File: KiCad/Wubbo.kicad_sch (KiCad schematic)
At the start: 43 parts, among them J1 USB_C_Receptacle, J2 SWD, J3 USB, J4 JST-BATT, Q1 AO3407, Q2 AO3407, SW1 Choc, SW10 Choc, SW11 Choc, SW12 Choc, SW13 Choc, SW14 Choc, SW15 Choc, SW16 Choc, SW17 Choc, SW2 Choc, SW3 Choc, SW4 Choc, SW5 Choc, SW6 Choc, SW7 Choc, SW8 Choc, SW9 Choc, U1 nRF52840_holyiot_18010, U2 XC6206P LDO, U3 LTC4054ES5-4.2

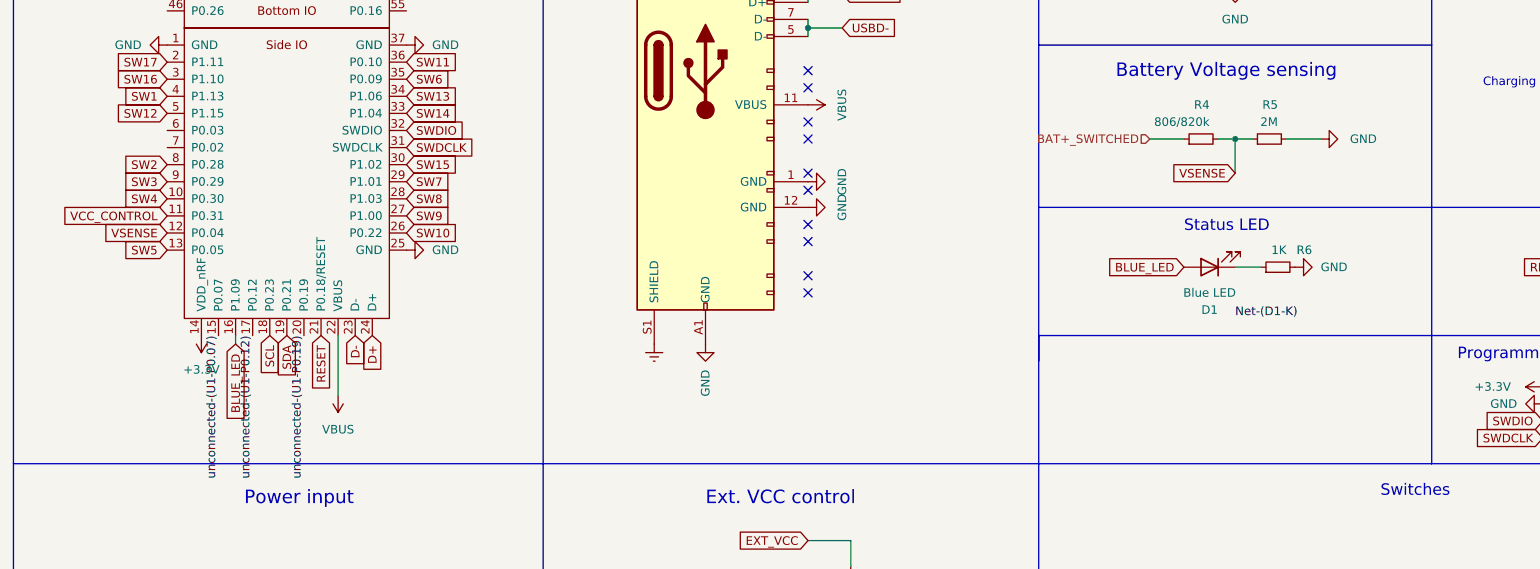
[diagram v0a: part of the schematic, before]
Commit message: WIP
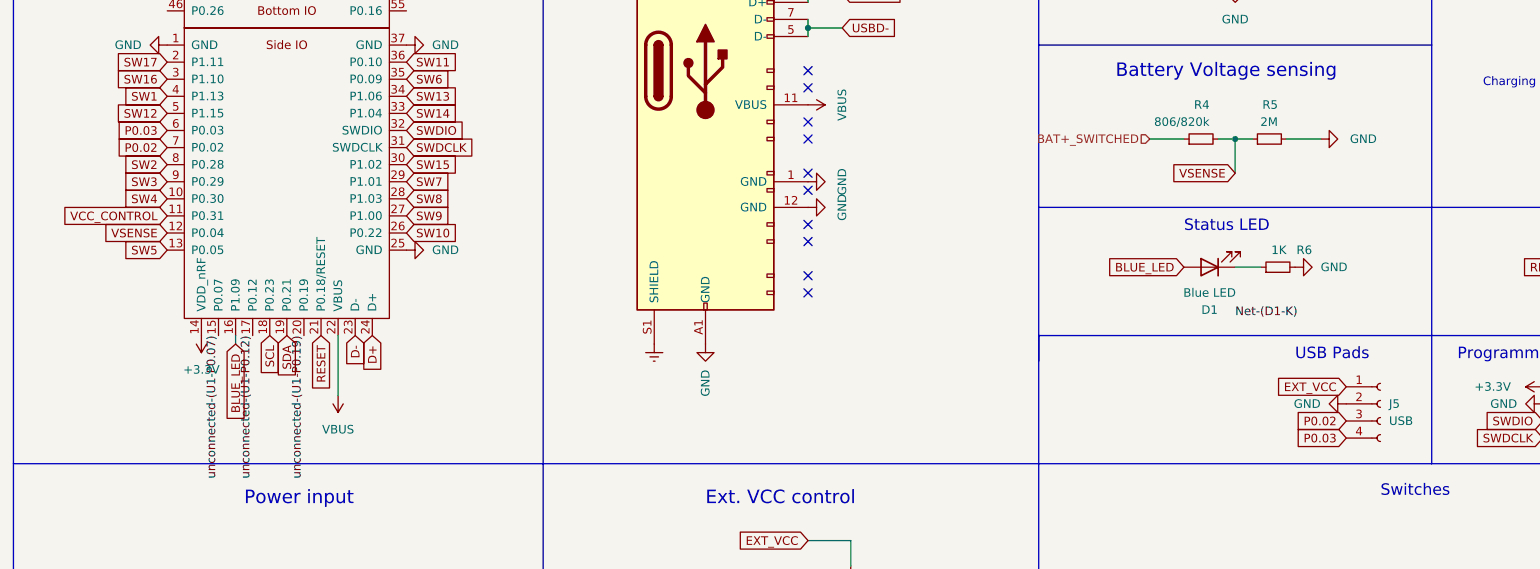
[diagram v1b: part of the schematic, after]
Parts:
- added J5: USB, Connector_PinHeader_2.00mm:PinHeader_1x04_P2.00mm_Vertical, symbol Connector:Conn_01x04_Female
- SW1, SW10, SW11, SW12, SW13, SW14, SW15, SW16, SW17, SW2, SW3, SW4, SW5, SW6, SW7, SW8, SW9: footprint kicad-keyboard-parts:PG13500-reversible -> kiboard_cache:PG13500-reversible
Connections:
- net EXT_VCC: now also J5.1 (Pin_1)
- net GND: now also J5.2 (Pin_2)
- net P0.03: now reaches U1.6 (P0.03)
- net P0.03: now also J5.4 (Pin_4)
- net P0.02: now reaches U1.7 (P0.02)
- net P0.02: now also J5.3 (Pin_3)

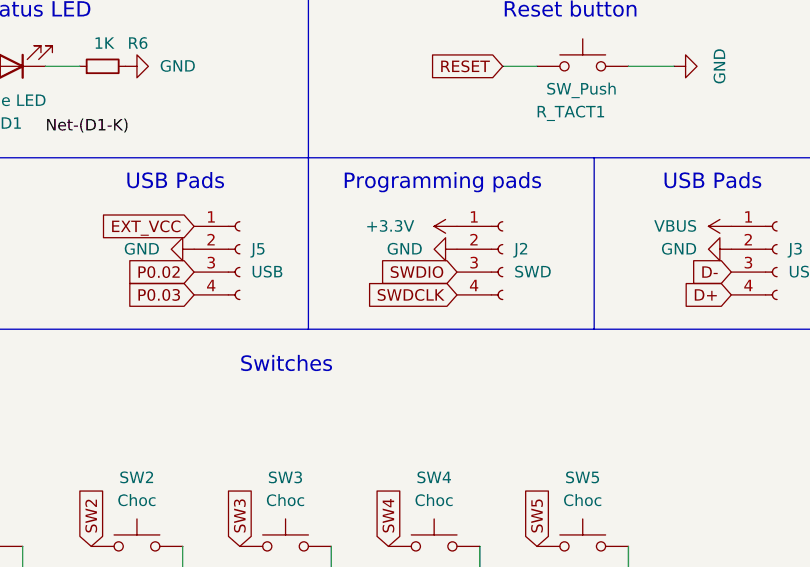
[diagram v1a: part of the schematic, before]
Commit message: WIP
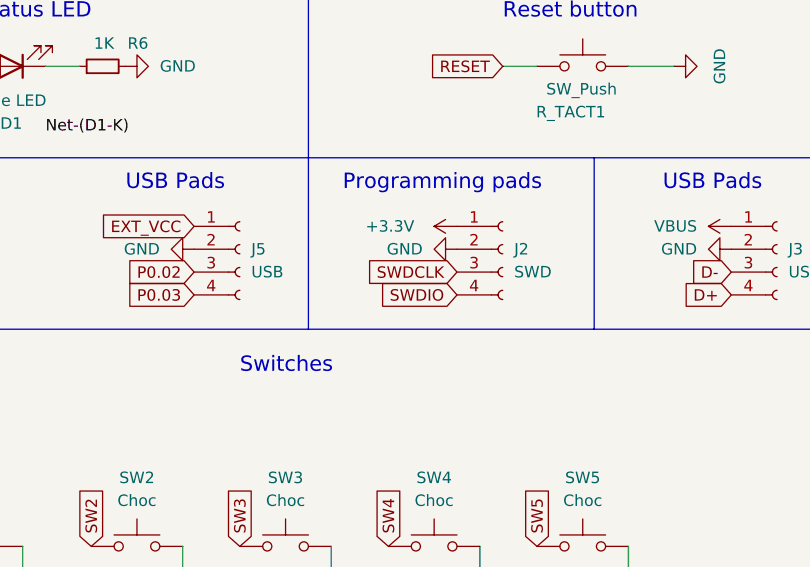
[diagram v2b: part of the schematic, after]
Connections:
- net SWDCLK: now also J2.3 (Pin_3); no longer J2.4 (Pin_4)
- net SWDIO: now also J2.4 (Pin_4); no longer J2.3 (Pin_3)
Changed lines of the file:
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@@
     )
   )
-  (global_label "SWDCLK" (shape input) (at 240.03 114.3 180) (fields_autoplaced)
-    (effects (font (size 1.27 1.27)) (justify right))
-    (property "Intersheet References" "${INTERSHEET_REFS}" (id 0) (at 230.2068 114.3794 0)
+  (global_label "SWDCLK" (shape input) (at 240.03 111.76 180) (fields_autoplaced)
+    (effects (font (size 1.27 1.27)) (justify right))
+    (property "Intersheet References" "${INTERSHEET_REFS}" (id 0) (at 230.2068 111.8394 0)
       (effects (font (size 1.27 1.27)) (justify right) hide)
     )
@@
     )
   )
-  (global_label "SWDIO" (shape input) (at 240.03 111.76 180) (fields_autoplaced)
-    (effects (font (size 1.27 1.27)) (justify right))
-    (property "Intersheet References" "${INTERSHEET_REFS}" (id 0) (at 231.8396 111.8394 0)
-      (effects (font (size 1.27 1.27)) (justify right) hide)
-    )
+  (global_label "SWDIO" (shape input) (at 240.03 114.3 180) (fields_autoplaced)
+    (effects (font (size 1.27 1.27)) (justify right))
+    (property "Intersheet References" "${INTERSHEET_REFS}" (id 0) (at 231.8396 114.3794 0)
+      (effects (font (size 1.27 1.27)) (justify right) hide)
+    )
